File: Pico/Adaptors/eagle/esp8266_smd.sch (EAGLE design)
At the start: 3 parts

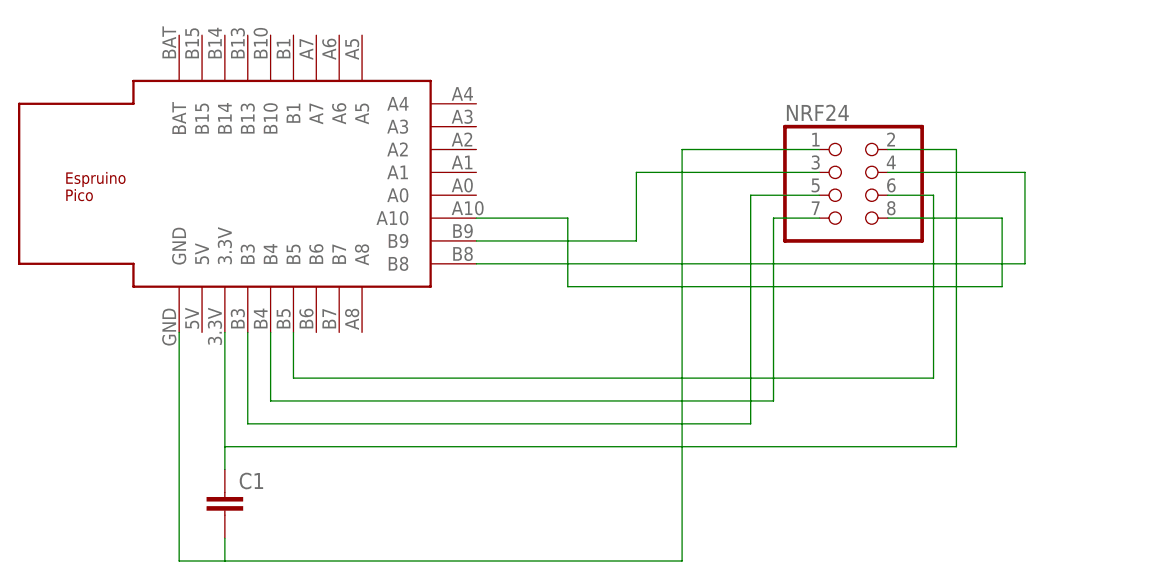
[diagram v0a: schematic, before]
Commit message: tweaking
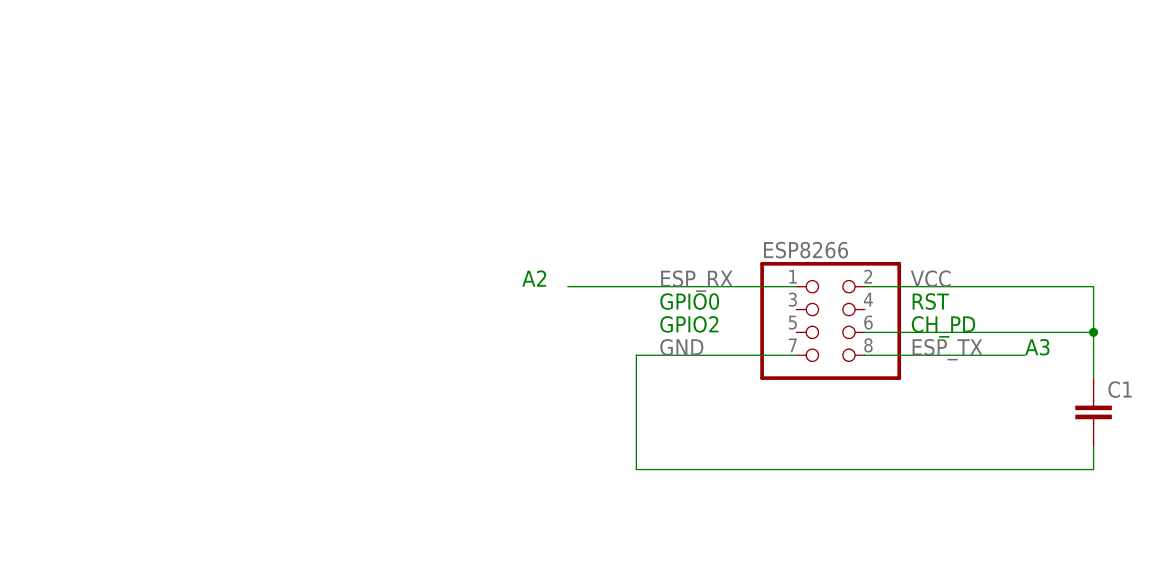
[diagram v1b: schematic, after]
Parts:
- removed NRF24: (no value), pinhead:PINHD-2X4
- removed U$1: ESPRUINO_PICO_SMDONLY, espruino_pico:ESPRUINO_PICO_SMDONLY
- added ESP8266: (no value), pinhead:PINHD-2X4
- C1: device rcl:C-EUC1206 -> rcl:C-EUC1210
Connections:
- removed net N$1: C1.1, NRF24.2, U$1.3.3V
- removed net N$2: C1.2, NRF24.1, U$1.GND
- removed net N$4: NRF24.5, U$1.B3
- removed net N$5: NRF24.7, U$1.B4
- removed net N$6: NRF24.6, U$1.B5
- removed net N$7: NRF24.4, U$1.B8
- removed net N$8: NRF24.3, U$1.B9
- removed net N$9: NRF24.8, U$1.A10
- new net ESP_RX: ESP8266.1
- new net ESP_TX: ESP8266.8
- new net GND: C1.2, ESP8266.7
- new net VCC: C1.1, ESP8266.2, ESP8266.6
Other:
- note added: "A2"
- note added: "A3"
- note added: "CH_PD"
- note added: "GPIO0"
- note added: "GPIO2"
- note added: "RST"
- moved on the sheet: C1
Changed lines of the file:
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@@
 </classes>
 <parts>
-<part name="NRF24" library="pinhead" deviceset="PINHD-2X4" device=""/>
-<part name="C1" library="rcl" deviceset="C-EU" device="C1206"/>
-<part name="U$1" library="espruino_pico" deviceset="ESPRUINO_PICO_SMDONLY" device=""/>
+<part name="ESP8266" library="pinhead" deviceset="PINHD-2X4" device=""/>
+<part name="C1" library="rcl" deviceset="C-EU" device="C1210"/>
 </parts>
 <sheets>
 <sheet>
 <plain>
+<text x="106.68" y="40.64" size="1.778" layer="91">CH_PD</text>
+<text x="106.68" y="43.18" size="1.778" layer="91">RST</text>
+<text x="78.74" y="43.18" size="1.778" layer="91">GPIO0</text>
+<text x="78.74" y="40.64" size="1.778" layer="91">GPIO2</text>
+<text x="63.5" y="45.72" size="1.778" layer="91">A2</text>
+<text x="119.38" y="38.1" size="1.778" layer="91">A3</text>
 </plain>
 <instances>
-<instance part="NRF24" gate="A" x="99.06" y="55.88"/>
-<instance part="C1" gate="G$1" x="30.48" y="22.86"/>
-<instance part="U$1" gate="G$1" x="33.02" y="66.04"/>
+<instance part="ESP8266" gate="A" x="96.52" y="40.64"/>
+<instance part="C1" gate="G$1" x="127" y="33.02"/>
 </instances>
 <busses>
 </busses>
 <nets>
-<net name="N$1" class="0">
+<net name="ESP_RX" class="0">
 <segment>
-<pinref part="C1" gate="G$1" pin="1"/>
-<wire x1="30.48" y1="40.64" x2="30.48" y2="27.94" width="0.1524" layer="91"/>
-<pinref part="NRF24" gate="A" pin="2"/>
-<wire x1="30.48" y1="27.94" x2="30.48" y2="25.4" width="0.1524" layer="91"/>
-<wire x1="104.14" y1="60.96" x2="111.76" y2="60.96" width="0.1524" layer="91"/>
-<wire x1="111.76" y1="60.96" x2="111.76" y2="27.94" width="0.1524" layer="91"/>
-<wire x1="111.76" y1="27.94" x2="30.48" y2="27.94" width="0.1524" layer="91"/>
-<pinref part="U$1" gate="G$1" pin="3.3V"/>
+<pinref part="ESP8266" gate="A" pin="1"/>
+<wire x1="93.98" y1="45.72" x2="68.58" y2="45.72" width="0.1524" layer="91"/>
+<label x="78.74" y="45.72" size="1.778" layer="95"/>
 </segment>
 </net>
-<net name="N$2" class="0">
+<net name="ESP_TX" class="0">
 <segment>
-<wire x1="25.4" y1="40.64" x2="25.4" y2="15.24" width="0.1524" layer="91"/>
-<wire x1="25.4" y1="15.24" x2="30.48" y2="15.24" width="0.1524" layer="91"/>
-<pinref part="C1" gate="G$1" pin="2"/>
-<wire x1="30.48" y1="15.24" x2="30.48" y2="17.78" width="0.1524" layer="91"/>
-<wire x1="30.48" y1="15.24" x2="81.28" y2="15.24" width="0.1524" layer="91"/>
-<wire x1="81.28" y1="15.24" x2="81.28" y2="60.96" width="0.1524" layer="91"/>
-<pinref part="NRF24" gate="A" pin="1"/>
-<wire x1="81.28" y1="60.96" x2="96.52" y2="60.96" width="0.1524" layer="91"/>
-<pinref part="U$1" gate="G$1" pin="GND"/>
+<pinref part="ESP8266" gate="A" pin="8"/>
+<wire x1="101.6" y1="38.1" x2="119.38" y2="38.1" width="0.1524" layer="91"/>
+<label x="106.68" y="38.1" size="1.778" layer="95"/>
 </segment>
 </net>
-<net name="N$4" class="0">
+<net name="VCC" class="0">
 <segment>
-<wire x1="33.02" y1="40.64" x2="33.02" y2="30.48" width="0.1524" layer="91"/>
-<wire x1="33.02" y1="30.48" x2="88.9" y2="30.48" width="0.1524" layer="91"/>
-<wire x1="88.9" y1="30.48" x2="88.9" y2="55.88" width="0.1524" layer="91"/>
-<pinref part="NRF24" gate="A" pin="5"/>
-<wire x1="88.9" y1="55.88" x2="96.52" y2="55.88" width="0.1524" layer="91"/>
-<pinref part="U$1" gate="G$1" pin="B3"/>
+<pinref part="ESP8266" gate="A" pin="2"/>
+<wire x1="101.6" y1="45.72" x2="127" y2="45.72" width="0.1524" layer="91"/>
+<wire x1="127" y1="45.72" x2="127" y2="40.64" width="0.1524" layer="91"/>
+<wire x1="127" y1="40.64" x2="127" y2="35.56" width="0.1524" layer="91"/>
+<label x="106.68" y="45.72" size="1.778" layer="95"/>
+<pinref part="ESP8266" gate="A" pin="6"/>
+<wire x1="101.6" y1="40.64" x2="127" y2="40.64" width="0.1524" layer="91"/>
+<junction x="127" y="40.64"/>
+<pinref part="C1" gate="G$1" pin="1"/>
 </segment>
 </net>
-<net name="N$5" class="0">
+<net name="GND" class="0">
 <segment>
-<pinref part="NRF24" gate="A" pin="7"/>
-<wire x1="96.52" y1="53.34" x2="91.44" y2="53.34" width="0.1524" layer="91"/>
-<wire x1="91.44" y1="53.34" x2="91.44" y2="33.02" width="0.1524" layer="91"/>
-<wire x1="91.44" y1="33.02" x2="35.56" y2="33.02" width="0.1524" layer="91"/>
-<wire x1="35.56" y1="33.02" x2="35.56" y2="40.64" width="0.1524" layer="91"/>
-<pinref part="U$1" gate="G$1" pin="B4"/>
-</segment>
-</net>
-<net name="N$6" class="0">
-<segment>
-<wire x1="38.1" y1="40.64" x2="38.1" y2="35.56" width="0.1524" layer="91"/>
-<wire x1="38.1" y1="35.56" x2="109.22" y2="35.56" width="0.1524" layer="91"/>
-<wire x1="109.22" y1="35.56" x2="109.22" y2="55.88" width="0.1524" layer="91"/>
-<pinref part="NRF24" gate="A" pin="6"/>
-<wire x1="109.22" y1="55.88" x2="104.14" y2="55.88" width="0.1524" layer="91"/>
-<pinref part="U$1" gate="G$1" pin="B5"/>
-</segment>
-</net>
-<net name="N$7" class="0">
-<segment>
-<wire x1="58.42" y1="48.26" x2="119.38" y2="48.26" width="0.1524" layer="91"/>
-<wire x1="119.38" y1="48.26" x2="119.38" y2="58.42" width="0.1524" layer="91"/>
-<pinref part="NRF24" gate="A" pin="4"/>
-<wire x1="119.38" y1="58.42" x2="104.14" y2="58.42" width="0.1524" layer="91"/>
-<pinref part="U$1" gate="G$1" pin="B8"/>
-</segment>
-</net>
-<net name="N$8" class="0">
-<segment>
-<pinref part="NRF24" gate="A" pin="3"/>
-<wire x1="96.52" y1="58.42" x2="76.2" y2="58.42" width="0.1524" layer="91"/>
-<wire x1="76.2" y1="58.42" x2="76.2" y2="50.8" width="0.1524" layer="91"/>
-<wire x1="76.2" y1="50.8" x2="58.42" y2="50.8" width="0.1524" layer="91"/>
-<pinref part="U$1" gate="G$1" pin="B9"/>
-</segment>
-</net>
-<net name="N$9" class="0">
-<segment>
-<wire x1="58.42" y1="53.34" x2="68.58" y2="53.34" width="0.1524" layer="91"/>
-<wire x1="68.58" y1="53.34" x2="68.58" y2="45.72" width="0.1524" layer="91"/>
-<wire x1="68.58" y1="45.72" x2="116.84" y2="45.72" width="0.1524" layer="91"/>
-<wire x1="116.84" y1="45.72" x2="116.84" y2="53.34" width="0.1524" layer="91"/>
-<pinref part="NRF24" gate="A" pin="8"/>
-<wire x1="116.84" y1="53.34" x2="104.14" y2="53.34" width="0.1524" layer="91"/>
-<pinref part="U$1" gate="G$1" pin="A10"/>
+<wire x1="127" y1="25.4" x2="76.2" y2="25.4" width="0.1524" layer="91"/>
+<wire x1="76.2" y1="25.4" x2="76.2" y2="38.1" width="0.1524" layer="91"/>
+<pinref part="ESP8266" gate="A" pin="7"/>
+<wire x1="76.2" y1="38.1" x2="93.98" y2="38.1" width="0.1524" layer="91"/>
+<label x="78.74" y="38.1" size="1.778" layer="95"/>
+<pinref part="C1" gate="G$1" pin="2"/>
+<wire x1="127" y1="27.94" x2="127" y2="25.4" width="0.1524" layer="91"/>
 </segment>
 </net>
@@
 </schematic>
 </drawing>
-<compatibility>
-<note version="6.3" minversion="6.2.2" severity="warning">
-Since Version 6.2.2 text objects can contain more than one line,
-which will not be processed correctly with this version.
-</note>
-</compatibility>
 </eagle>
